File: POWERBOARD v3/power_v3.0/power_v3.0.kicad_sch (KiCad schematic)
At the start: 0 parts

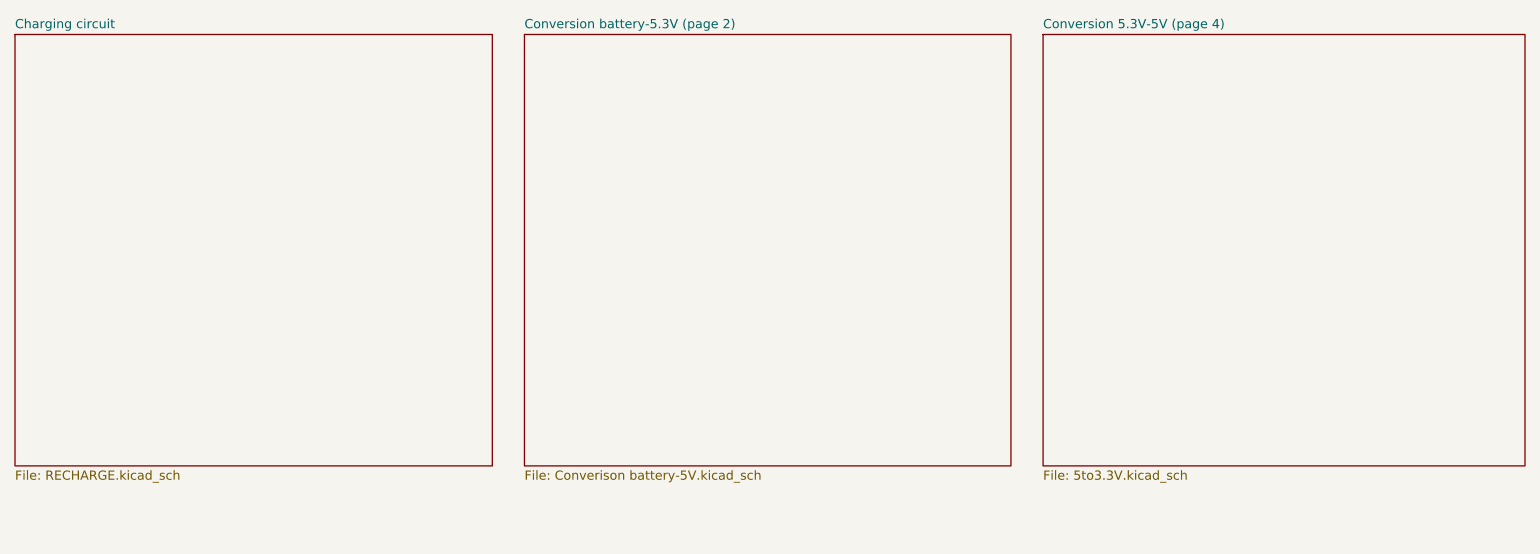
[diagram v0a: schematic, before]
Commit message: updated file names and added hierarchy schematic, problem with ERC bc of GND
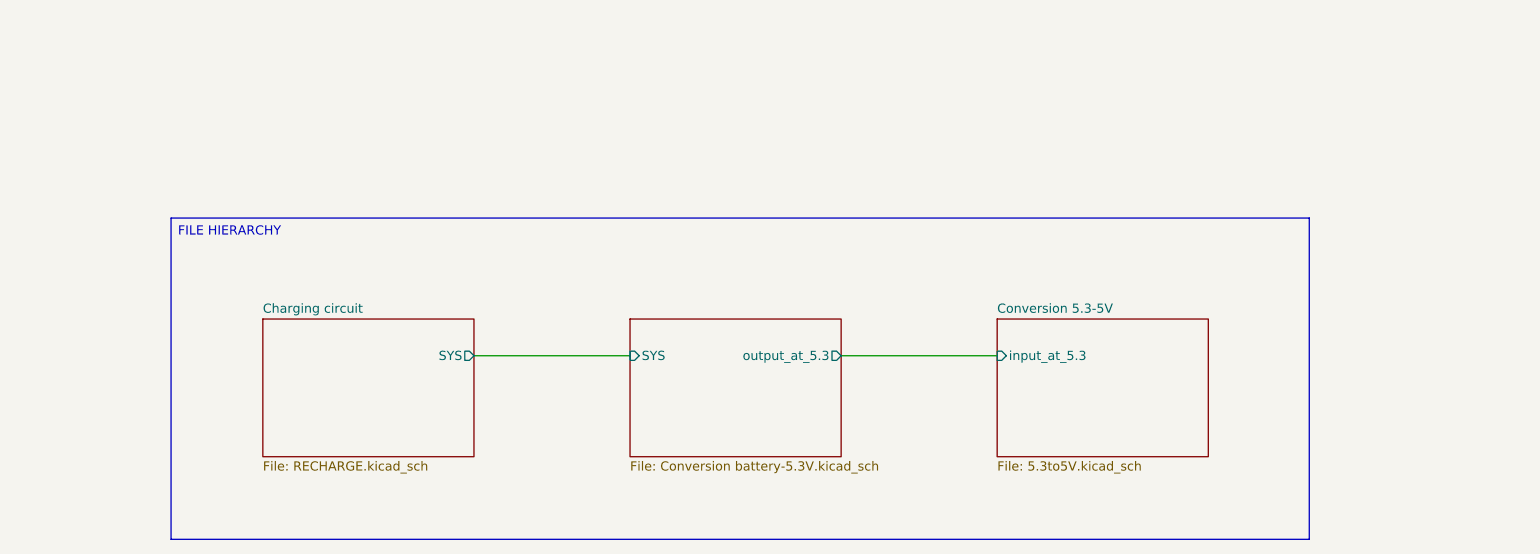
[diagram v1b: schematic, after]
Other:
- removed sheet Conversion 5.3V-5V (page 4)
- removed sheet Conversion battery-5.3V (page 2)
- added sheet Conversion 5.3-5V (5.3to5V.kicad_sch)
- added sheet Conversion battery-5.3V (Conversion battery-5.3V.kicad_sch)
- sheet Charging circuit ports: added SYS; removed none
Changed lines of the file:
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@@
 	(generator_version "10.0")
 	(paper "A4")
+	(text_box "FILE HIERARCHY"
+		(exclude_from_sim no)
+		(at 60.96 88.9 0)
+		(size 157.48 44.45)
+		(margins 0.9525 0.9525 0.9525 0.9525)
+		(stroke
+			(width 0)
+			(type solid)
+		)
+		(fill
+			(type none)
+		)
+		(effects
+			(font
+				(size 1.27 1.27)
+			)
+			(justify left top)
+		)
+	)
+	(wire
+		(pts
+			(xy 153.67 107.95) (xy 175.26 107.95)
+		)
+		(stroke
+			(width 0)
+			(type default)
+		)
+	)
+	(wire
+		(pts
+			(xy 102.87 107.95) (xy 124.46 107.95)
+		)
+		(stroke
+			(width 0)
+			(type default)
+		)
+	)
 	(sheet
-		(at 109.855 63.5)
-		(size 67.31 59.69)
+		(at 124.46 102.87)
+		(size 29.21 19.05)
 		(exclude_from_sim no)
 		(in_bom yes)
@@
 			(color 0 0 0 0)
 		)
-		(property "Sheetname" "Conversion battery-5.3V (page 2)"
-			(at 109.855 62.7884 0)
+		(property "Sheetname" "Conversion battery-5.3V"
+			(at 124.46 102.1584 0)
+			(hide yes)
 			(show_name no)
 			(do_not_autoplace no)
@@
 			)
 		)
-		(property "Sheetfile" "Converison battery-5V.kicad_sch"
-			(at 109.855 123.7746 0)
+		(property "Sheetfile" "Conversion battery-5.3V.kicad_sch"
+			(at 124.46 122.5046 0)
 			(show_name no)
 			(do_not_autoplace no)
@@
 				)
 				(justify left top)
+			)
+		)
+		(pin "SYS" input
+			(at 124.46 107.95 180)
+			(effects
+				(font
+					(size 1.27 1.27)
+				)
+				(justify left)
+			)
+		)
+		(pin "output_at_5.3" output
+			(at 153.67 107.95 0)
+			(effects
+				(font
+					(size 1.27 1.27)
+				)
+				(justify right)
 			)
 		)
@@
 	)
 	(sheet
-		(at 181.61 63.5)
-		(size 66.675 59.69)
+		(at 73.66 102.87)
+		(size 29.21 19.05)
 		(exclude_from_sim no)
 		(in_bom yes)
@@
 			(color 0 0 0 0)
 		)
-		(property "Sheetname" "Conversion 5.3V-5V (page 4)"
-			(at 181.61 62.7884 0)
+		(property "Sheetname" "Charging circuit"
+			(at 73.66 102.1584 0)
 			(show_name no)
 			(do_not_autoplace no)
@@
 			)
 		)
-		(property "Sheetfile" "5to3.3V.kicad_sch"
-			(at 181.61 123.7746 0)
+		(property "Sheetfile" "RECHARGE.kicad_sch"
+			(at 73.66 122.5046 0)
 			(show_name no)
 			(do_not_autoplace no)
@@
 				)
 				(justify left top)
+			)
+		)
+		(pin "SYS" output
+			(at 102.87 107.95 0)
+			(effects
+				(font
+					(size 1.27 1.27)
+				)
+				(justify right)
+			)
+		)
+		(instances
+			(project "power_v3.0"
+				(path "/432bcdcf-747a-4fa0-b87b-096f44260199"
+					(page "3")
+				)
+			)
+		)
+	)
+	(sheet
+		(at 175.26 102.87)
+		(size 29.21 19.05)
+		(exclude_from_sim no)
+		(in_bom yes)
+		(on_board yes)
+		(dnp no)
+		(fields_autoplaced yes)
+		(stroke
+			(width 0.1524)
+			(type solid)
+		)
+		(fill
+			(color 0 0 0 0)
+		)
+		(property "Sheetname" "Conversion 5.3-5V"
+			(at 175.26 102.1584 0)
+			(show_name no)
+			(do_not_autoplace no)
+			(effects
+				(font
+					(size 1.27 1.27)
+				)
+				(justify left bottom)
+			)
+		)
+		(property "Sheetfile" "5.3to5V.kicad_sch"
+			(at 175.26 122.5046 0)
+			(show_name no)
+			(do_not_autoplace no)
+			(effects
+				(font
+					(size 1.27 1.27)
+				)
+				(justify left top)
+			)
+		)
+		(pin "input_at_5.3" input
+			(at 175.26 107.95 180)
+			(effects
+				(font
+					(size 1.27 1.27)
+				)
+				(justify left)
 			)
 		)
@@
 				)
 			)
-		)
-	)
-	(sheet
-		(at 39.37 63.5)
-		(size 66.04 59.69)
-		(exclude_from_sim no)
-		(in_bom yes)
-		(on_board yes)
-		(dnp no)
-		(fields_autoplaced yes)
-		(stroke
-			(width 0.1524)
-			(type solid)
-		)
-		(fill
-			(color 0 0 0 0)
-		)
-		(property "Sheetname" "Charging circuit"
-			(at 39.37 62.7884 0)
-			(show_name no)
-			(do_not_autoplace no)
-			(effects
-				(font
-					(size 1.27 1.27)
-				)
-				(justify left bottom)
-			)
-		)
-		(property "Sheetfile" "RECHARGE.kicad_sch"
-			(at 39.37 123.7746 0)
-			(show_name no)
-			(do_not_autoplace no)
-			(effects
-				(font
-					(size 1.27 1.27)
-				)
-				(justify left top)
-			)
-		)
-		(instances
-			(project "power_v3.0"
-				(path "/432bcdcf-747a-4fa0-b87b-096f44260199"
-					(page "3")
-				)
-			)
